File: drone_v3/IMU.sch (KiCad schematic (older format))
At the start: 24 parts, among them J2 Conn_01x10_Female, U10 ICM-20948, U3 MPU-9250, U4 MCP1700-3302E_SOT23, U7 BMP280, U8 MCP1804x-1802xDB

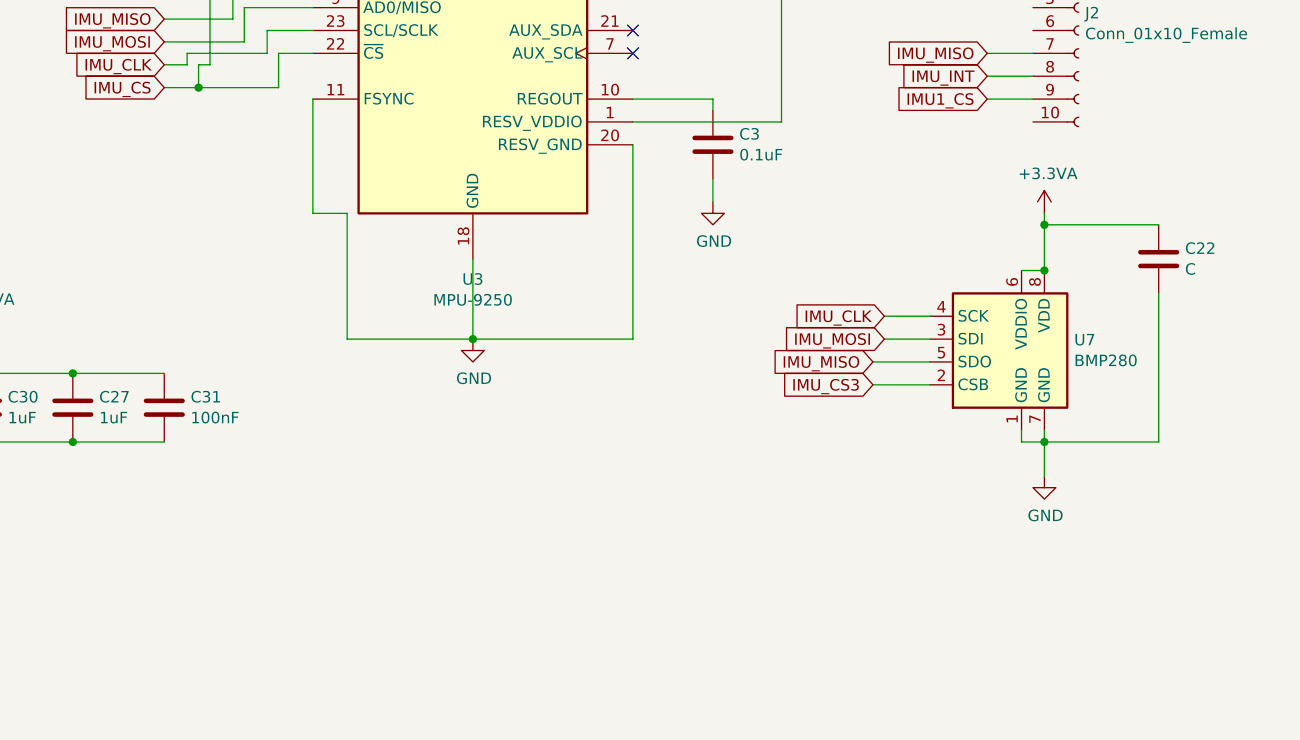
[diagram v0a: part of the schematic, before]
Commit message: add alot
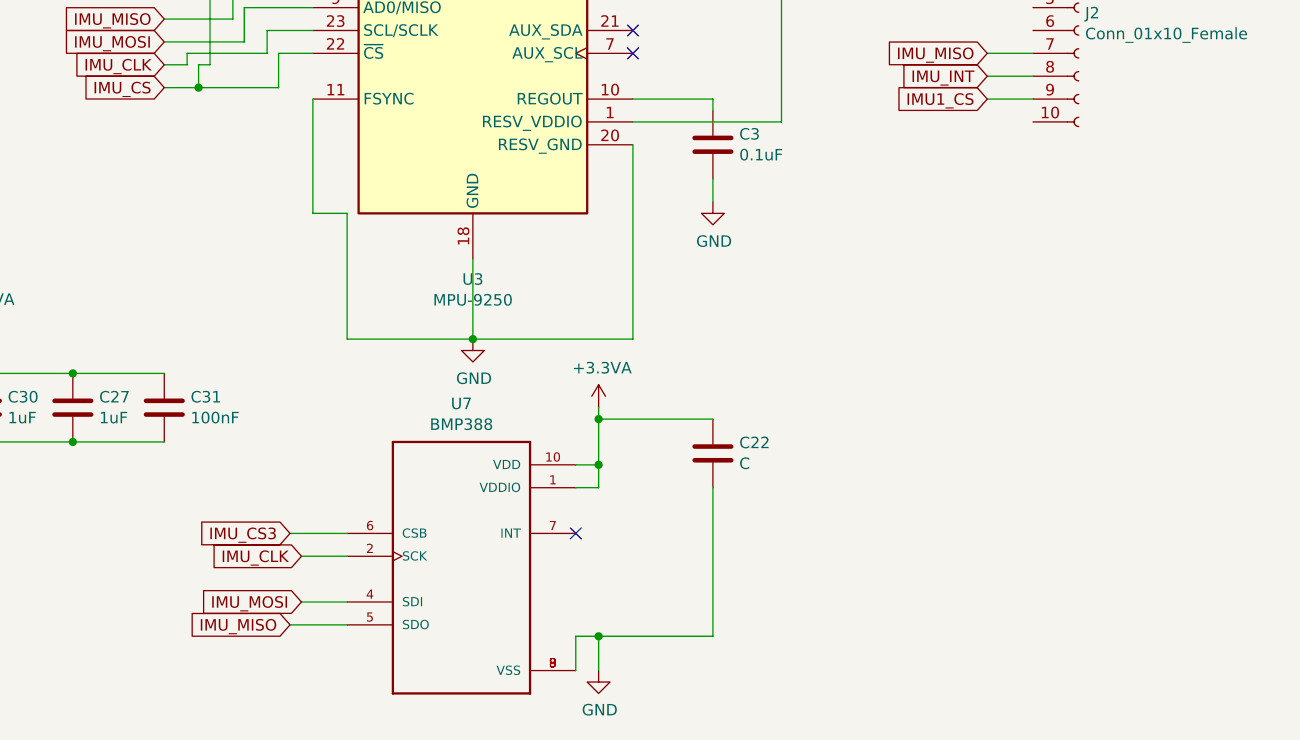
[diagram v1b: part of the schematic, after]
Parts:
- removed U7: BMP280, Package_LGA:Bosch_LGA-8_2x2.5mm_P0.65mm_ClockwisePinNumbering, symbol Sensor_Pressure:BMP280
- added U7: BMP388, PQFN50P200X200X80-10N, symbol bmp388:BMP388
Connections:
- net +3.3VA: now also U7.1 (VDDIO), U7.10 (VDD)
- net GND: now also U7.3 (VSS), U7.8 (VSS), U7.9 (VSS)
- net IMU_CLK: now also U7.2 (SCK)
- net IMU_CS3: now also U7.6 (CSB)
- net IMU_MISO: now also U7.5 (SDO)
- net IMU_MOSI: now also U7.4 (SDI)
- no-connect marks 4 -> 5
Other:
- moved on the sheet: C22
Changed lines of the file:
@@
 Wire Wire Line
 	6600 5550 5900 5550
-Text GLabel 7700 5450 0    50   Input ~ 0
+Text GLabel 5150 6500 0    50   Input ~ 0
 IMU_CLK
-Text GLabel 7700 5550 0    50   Input ~ 0
+Text GLabel 5150 6700 0    50   Input ~ 0
 IMU_MOSI
-Text GLabel 7650 5650 0    50   Input ~ 0
+Text GLabel 5100 6800 0    50   Input ~ 0
 IMU_MISO
 Wire Wire Line
-	7700 5550 7900 5550
-Wire Wire Line
-	7650 5650 7900 5650
-Wire Wire Line
-	7700 5450 7900 5450
-Wire Wire Line
-	8400 5000 8400 5050
-Wire Wire Line
-	8400 5950 8400 6000
+	5150 6700 5350 6700
+Wire Wire Line
+	5100 6800 5350 6800
+Wire Wire Line
+	5150 6500 5350 6500
+Wire Wire Line
+	6450 5850 6450 5900
 $Comp
 L power:GND #PWR0140
 U 1 1 5F2FBD71
-P 8400 6150
-F 0 "#PWR0140" H 8400 5900 50  0001 C CNN
-F 1 "GND" H 8405 5977 50  0000 C CNN
-F 2 "" H 8400 6150 50  0001 C CNN
-F 3 "" H 8400 6150 50  0001 C CNN
-	1    8400 6150
+P 6450 7000
+F 0 "#PWR0140" H 6450 6750 50  0001 C CNN
+F 1 "GND" H 6455 6827 50  0000 C CNN
+F 2 "" H 6450 7000 50  0001 C CNN
+F 3 "" H 6450 7000 50  0001 C CNN
+	1    6450 7000
 	1    0    0    -1
 $EndComp
@@
 L Device:C C22
 U 1 1 5F2FCC1C
-P 8900 5200
-F 0 "C22" H 9015 5246 50  0000 L CNN
-F 1 "C" H 9015 5155 50  0000 L CNN
-F 2 "Capacitor_SMD:C_0603_1608Metric" H 8938 5050 50  0001 C CNN
-F 3 "~" H 8900 5200 50  0001 C CNN
-	1    8900 5200
-	1    0    0    -1
-$EndComp
-Wire Wire Line
-	8400 5050 8900 5050
-Connection ~ 8400 5050
-Wire Wire Line
-	8900 5350 8900 6000
-Wire Wire Line
-	8900 6000 8400 6000
-Connection ~ 8400 6000
-Wire Wire Line
-	8400 6000 8400 6150
+P 6950 6050
+F 0 "C22" H 7065 6096 50  0000 L CNN
+F 1 "C" H 7065 6005 50  0000 L CNN
+F 2 "Capacitor_SMD:C_0603_1608Metric" H 6988 5900 50  0001 C CNN
+F 3 "~" H 6950 6050 50  0001 C CNN
+	1    6950 6050
+	1    0    0    -1
+$EndComp
+Wire Wire Line
+	6450 5900 6950 5900
+Connection ~ 6450 5900
+Wire Wire Line
+	6950 6200 6950 6850
+Wire Wire Line
+	6950 6850 6450 6850
+Connection ~ 6450 6850
+Wire Wire Line
+	6450 6850 6450 7000
 Wire Wire Line
 	2050 1250 2050 1650
@@
 Text GLabel 1200 2350 0    50   Input ~ 0
 IMU_CS2
-Text GLabel 7650 5750 0    50   Input ~ 0
+Text GLabel 5100 6400 0    50   Input ~ 0
 IMU_CS3
 Wire Wire Line
-	7650 5750 7900 5750
+	5100 6400 5350 6400
 $Comp
 L Device:CP C21
@@
 L power:+3.3VA #PWR0173
 U 1 1 5F38A5F4
-P 8400 5000
-F 0 "#PWR0173" H 8400 4850 50  0001 C CNN
-F 1 "+3.3VA" H 8415 5173 50  0000 C CNN
-F 2 "" H 8400 5000 50  0001 C CNN
-F 3 "" H 8400 5000 50  0001 C CNN
-	1    8400 5000
+P 6450 5850
+F 0 "#PWR0173" H 6450 5700 50  0001 C CNN
+F 1 "+3.3VA" H 6465 6023 50  0000 C CNN
+F 2 "" H 6450 5850 50  0001 C CNN
+F 3 "" H 6450 5850 50  0001 C CNN
+	1    6450 5850
 	1    0    0    -1
 $EndComp
@@
 	1    0    0    -1
 $EndComp
-$Comp
-L Sensor_Pressure:BMP280 U7
-U 1 1 5F412E16
-P 8300 5650
-F 0 "U7" H 8530 5746 50  0000 L CNN
-F 1 "BMP280" H 8530 5655 50  0000 L CNN
-F 2 "Package_LGA:Bosch_LGA-8_2x2.5mm_P0.65mm_ClockwisePinNumbering" H 8300 4950 50  0001 C CNN
-F 3 "https://ae-bst.resource.bosch.com/media/_tech/media/datasheets/BST-BMP280-DS001.pdf" H 8300 5650 50  0001 C CNN
-	1    8300 5650
-	1    0    0    -1
-$EndComp
-Wire Wire Line
-	8300 5250 8400 5250
-Wire Wire Line
-	8400 5050 8400 5250
-Connection ~ 8400 5250
-Wire Wire Line
-	8400 6000 8300 6000
-Wire Wire Line
-	8300 6000 8300 5950
+Wire Wire Line
+	6350 6100 6450 6100
+Wire Wire Line
+	6450 5900 6450 6100
 $Comp
 L Device:R R16
@@
 Wire Wire Line
 	5850 3250 5850 3300
+Wire Wire Line
+	6350 7000 6350 6850
+$Comp
+L bmp388:BMP388 U7
+U 1 1 5F504600
+P 5850 6600
+F 0 "U7" H 5850 7367 50  0000 C CNN
+F 1 "BMP388" H 5850 7276 50  0000 C CNN
+F 2 "PQFN50P200X200X80-10N" H 5850 6600 50  0001 L BNN
+F 3 "None" H 5850 6600 50  0001 L BNN
+F 4 "https://snapeda.com/shop?store=Mouser&id=2747857" H 5850 6600 50  0001 L BNN "Field4"
+F 5 "Bosch Sensortec" H 5850 6600 50  0001 L BNN "Field5"
+F 6 "https://snapeda.com/shop?store=DigiKey&id=2747857" H 5850 6600 50  0001 L BNN "Field6"
+F 7 "Pressure Sensor 4.35PSI ~ 18.13PSI (30kPa ~ 125kPa) Absolute 10-WFLGA" H 5850 6600 50  0001 L BNN "Field7"
+F 8 "WFLGA-10 Bosch Tools" H 5850 6600 50  0001 L BNN "Field8"
+F 9 "Warning" H 5850 6600 50  0001 L BNN "Field9"
+F 10 "BMP388" H 5850 6600 50  0001 L BNN "Field10"
+	1    5850 6600
+	1    0    0    -1
+$EndComp
+Wire Wire Line
+	6350 6850 6450 6850
+Wire Wire Line
+	6350 6200 6450 6200
+Wire Wire Line
+	6450 6200 6450 6100
+Connection ~ 6450 6100
+NoConn ~ 6350 6400
 $EndSCHEMATC

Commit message: fix alot
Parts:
- U7: symbol bmp388:BMP388 -> BMP388:BMP388
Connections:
- net IMU1_CS: now also U7.6 (CSB); no longer J2.9 (Pin_9)
- net IMU_CS3: now also J2.9 (Pin_9); no longer U7.6 (CSB)
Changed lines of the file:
@@
 Text GLabel 8150 4400 0    50   Input ~ 0
 IMU_INT
-Text GLabel 8150 4500 0    50   Input ~ 0
-IMU1_CS
 Wire Wire Line
 	8150 3800 8350 3800
@@
 Wire Wire Line
 	8150 4400 8350 4400
-Wire Wire Line
-	8350 4500 8150 4500
 $Comp
 L Device:R R1
@@
 Text GLabel 1200 2350 0    50   Input ~ 0
 IMU_CS2
-Text GLabel 5100 6400 0    50   Input ~ 0
-IMU_CS3
-Wire Wire Line
-	5100 6400 5350 6400
 $Comp
 L Device:CP C21
@@
 	6350 7000 6350 6850
 $Comp
-L bmp388:BMP388 U7
+L BMP388:BMP388 U7
 U 1 1 5F504600
 P 5850 6600
+AR Path="/5F504600" Ref="U7"  Part="1"
+AR Path="/5F3218EE/5F504600" Ref="U7"  Part="1"
 F 0 "U7" H 5850 7367 50  0000 C CNN
 F 1 "BMP388" H 5850 7276 50  0000 C CNN
@@
 Connection ~ 6450 6100
 NoConn ~ 6350 6400
+Wire Wire Line
+	8100 4500 8350 4500
+Text GLabel 8100 4500 0    50   Input ~ 0
+IMU_CS3
+Wire Wire Line
+	5350 6400 5150 6400
+Text GLabel 5150 6400 0    50   Input ~ 0
+IMU1_CS
 $EndSCHEMATC
